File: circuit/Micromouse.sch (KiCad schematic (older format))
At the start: 34 parts, among them J1 DBG_CN, J3 TEST_1P, J5 TEST_1P, J6 Conn_01x04, Q2 IRLML6344, SW2 SW_Push, SW3 SW_Push, SW4 SW_Push, U3 STM32F405RGTx, U7 ICM-20602-module

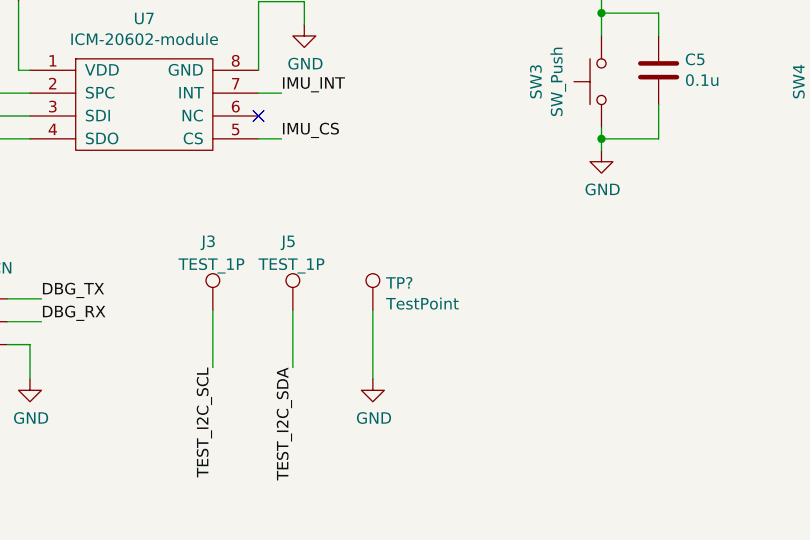
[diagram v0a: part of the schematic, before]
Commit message: AW終わったああああああああああああああ（はず）
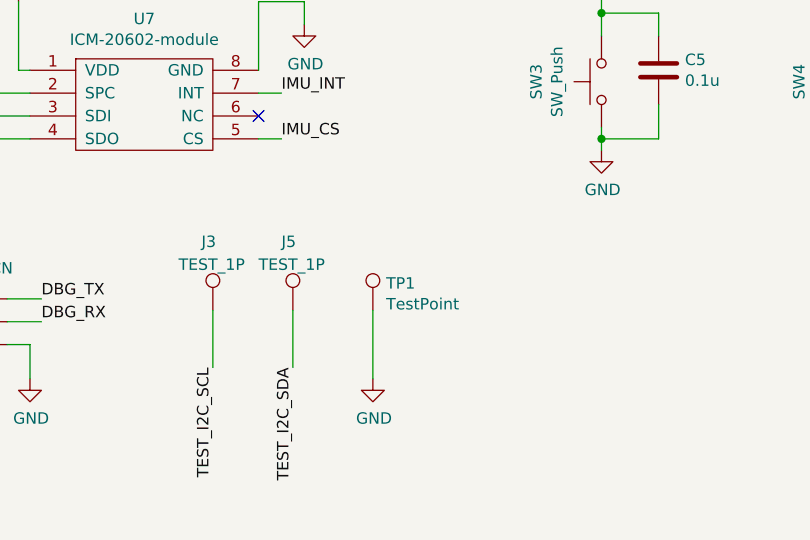
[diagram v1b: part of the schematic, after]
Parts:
- TP1: renamed from TP?; footprint (none) -> TestPoint:TestPoint_Pad_D1.0mm
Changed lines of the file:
@@
 	9250 6000 9450 6000
 $Comp
-L Connector:TestPoint TP?
+L Connector:TestPoint TP1
 U 1 1 5FFC074B
 P 6500 9800
-F 0 "TP?" H 6558 9918 50  0000 L CNN
+F 0 "TP1" H 6558 9918 50  0000 L CNN
 F 1 "TestPoint" H 6558 9827 50  0000 L CNN
-F 2 "" H 6700 9800 50  0001 C CNN
+F 2 "TestPoint:TestPoint_Pad_D1.0mm" H 6700 9800 50  0001 C CNN
 F 3 "~" H 6700 9800 50  0001 C CNN
 	1    6500 9800
@@
 $EndComp
 $Comp
-L power:GND #PWR?
+L power:GND #PWR0149
 U 1 1 5FFC282D
 P 6500 10100
-F 0 "#PWR?" H 6500 9850 50  0001 C CNN
+F 0 "#PWR0149" H 6500 9850 50  0001 C CNN
 F 1 "GND" H 6505 9927 50  0000 C CNN
 F 2 "" H 6500 10100 50  0001 C CNN
